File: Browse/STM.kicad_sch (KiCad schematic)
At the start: 2 parts

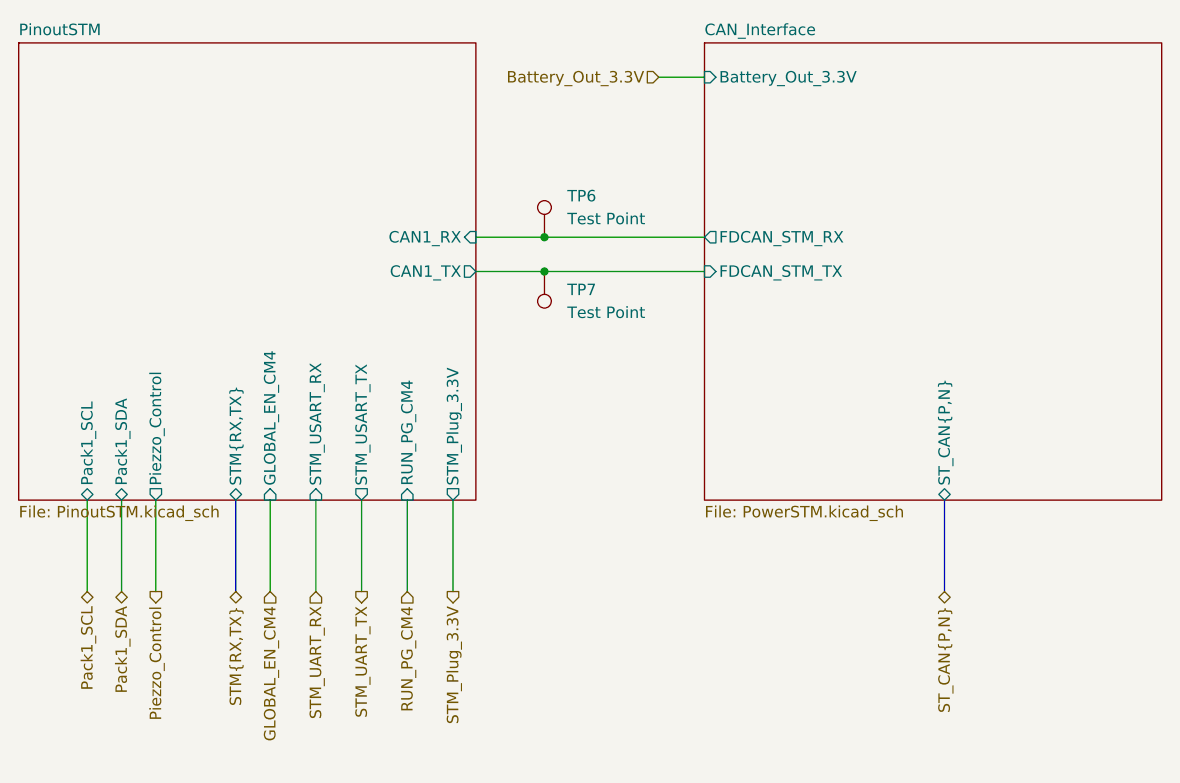
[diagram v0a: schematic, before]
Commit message: Deploying to gh-pages from @ Nautilus-UUV/nautilus-mainboard-PCB@5f5fdd9436d408a604bb268d740c0ac7ce1f5af5 🚀
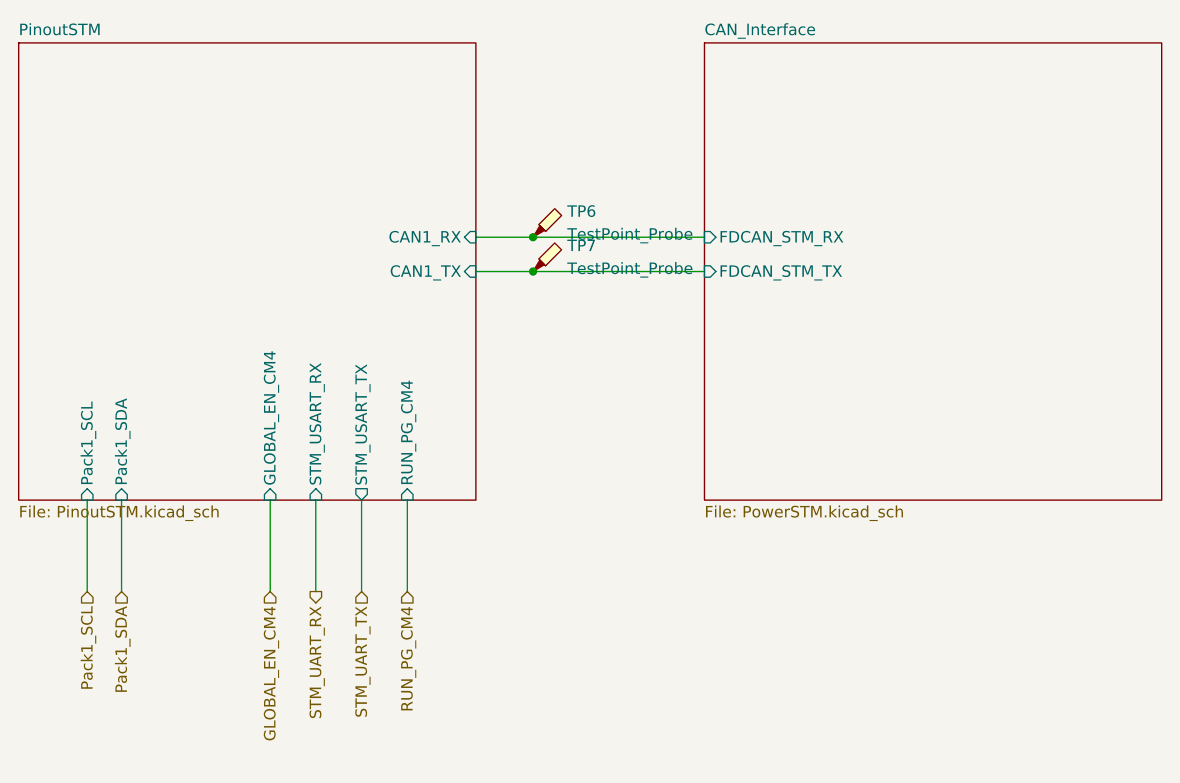
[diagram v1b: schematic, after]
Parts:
- removed TP6, TP7: Test Point, TestPoint:TestPoint_Pad_D1.5mm, symbol #dzdb:g_mech/M-TEST-SMT_1.5mm_round
- added TP6, TP7: TestPoint_Probe, TestPoint:TestPoint_THTPad_D2.5mm_Drill1.2mm, symbol Connector:TestPoint_Probe
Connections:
- net CAN_Interface/FDCAN_STM_RX: now also TP6.1
- net CAN_Interface/FDCAN_STM_TX: now also TP7.1
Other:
- sheet CAN_Interface ports: added none; removed Battery_Out_3.3V, ST_CAN{P,N}
- sheet PinoutSTM ports: added none; removed Piezzo_Control, STM_Plug_3.3V, STM{RX,TX}
- company: Evan -> (none)
- title: Nautilus_Mainboard -> (none)
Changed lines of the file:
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@@
 (kicad_sch (version 20250114) (generator "eeschema") (generator_version "9.0")
   (paper "A4")
-  (title_block
-    (title "Nautilus_Mainboard")
-    (date "2025-11-19")
-    (rev "0")
-    (company "Evan")
+  (junction (at 82.55 50.8) (diameter 0) (color 0 0 0 0)
   )
-  (junction (at 83.82 46.99) (diameter 0) (color 0 0 0 0)
+  (junction (at 82.55 46.99) (diameter 0) (color 0 0 0 0)
   )
-  (junction (at 83.82 50.8) (diameter 0) (color 0 0 0 0)
+  (wire (pts (xy 76.2 46.99) (xy 82.55 46.99))
+    (stroke (width 0) (type default))
   )
   (wire (pts (xy 63.5 76.2) (xy 63.5 86.36))
-    (stroke (width 0) (type default))
-  )
-  (bus (pts (xy 49.53 76.2) (xy 49.53 86.36))
-    (stroke (width 0) (type default))
-  )
-  (wire (pts (xy 40.64 76.2) (xy 40.64 86.36))
     (stroke (width 0) (type default))
   )
@@
     (stroke (width 0) (type default))
   )
-  (wire (pts (xy 73.66 76.2) (xy 73.66 86.36))
+  (wire (pts (xy 76.2 50.8) (xy 82.55 50.8))
     (stroke (width 0) (type default))
   )
-  (wire (pts (xy 76.2 46.99) (xy 83.82 46.99))
+  (wire (pts (xy 82.55 46.99) (xy 101.6 46.99))
     (stroke (width 0) (type default))
   )
@@
     (stroke (width 0) (type default))
   )
-  (wire (pts (xy 83.82 46.99) (xy 101.6 46.99))
-    (stroke (width 0) (type default))
-  )
   (wire (pts (xy 58.42 76.2) (xy 58.42 86.36))
     (stroke (width 0) (type default))
   )
-  (wire (pts (xy 83.82 50.8) (xy 101.6 50.8))
-    (stroke (width 0) (type default))
-  )
-  (bus (pts (xy 128.27 76.2) (xy 128.27 86.36))
-    (stroke (width 0) (type default))
-  )
-  (wire (pts (xy 96.52 29.21) (xy 101.6 29.21))
-    (stroke (width 0) (type default))
-  )
-  (wire (pts (xy 76.2 50.8) (xy 83.82 50.8))
+  (wire (pts (xy 82.55 50.8) (xy 101.6 50.8))
     (stroke (width 0) (type default))
   )
@@
     (stroke (width 0) (type default))
   )
-  (hierarchical_label "STM_UART_TX" (shape output) (at 63.5 86.36 270)
+  (hierarchical_label "STM_UART_TX" (shape input) (at 63.5 86.36 270)
     (effects (font (size 1.27 1.27)) (justify right))
   )
-  (hierarchical_label "STM_UART_RX" (shape input) (at 58.42 86.36 270)
+  (hierarchical_label "STM_UART_RX" (shape output) (at 58.42 86.36 270)
     (effects (font (size 1.27 1.27)) (justify right))
   )
@@
     (effects (font (size 1.27 1.27)) (justify right))
   )
-  (hierarchical_label "Pack1_SCL" (shape bidirectional) (at 33.02 86.36 270)
+  (hierarchical_label "Pack1_SCL" (shape input) (at 33.02 86.36 270)
     (effects (font (size 1.27 1.27)) (justify right))
   )
-  (hierarchical_label "STM{RX,TX}" (shape bidirectional) (at 49.53 86.36 270)
-    (effects (font (size 1.27 1.27)) (justify right))
-  )
-  (hierarchical_label "Battery_Out_3.3V" (shape input) (at 96.52 29.21 180)
-    (effects (font (size 1.27 1.27)) (justify right))
-  )
-  (hierarchical_label "STM_Plug_3.3V" (shape output) (at 73.66 86.36 270)
-    (effects (font (size 1.27 1.27)) (justify right))
-  )
-  (hierarchical_label "Piezzo_Control" (shape output) (at 40.64 86.36 270)
-    (effects (font (size 1.27 1.27)) (justify right))
-  )
-  (hierarchical_label "Pack1_SDA" (shape bidirectional) (at 36.83 86.36 270)
+  (hierarchical_label "Pack1_SDA" (shape input) (at 36.83 86.36 270)
     (effects (font (size 1.27 1.27)) (justify right))
   )
@@
     (effects (font (size 1.27 1.27)) (justify right))
   )
-  (hierarchical_label "ST_CAN{P,N}" (shape bidirectional) (at 128.27 86.36 270)
-    (effects (font (size 1.27 1.27)) (justify right))
-  )
-  (symbol (lib_id "#dzdb:g_mech/M-TEST-SMT_1.5mm_round") (at 83.82 46.99 0) (unit 1)
+  (symbol (lib_id "Connector:TestPoint_Probe") (at 82.55 46.99 0) (unit 1)
     (exclude_from_sim no) (in_bom yes) (on_board yes) (dnp no) (fields_autoplaced)
-    (property "Reference" "TP6" (at 86.36 42.4179 0)
+    (property "Reference" "TP6" (at 86.36 44.1324 0)
       (effects (font (size 1.27 1.27)) (justify left))
     )
-    (property "Value" "Test Point" (at 86.36 44.9579 0)
+    (property "Value" "TestPoint_Probe" (at 86.36 46.6724 0)
       (effects (font (size 1.27 1.27)) (justify left))
     )
-    (property "Footprint" "TestPoint:TestPoint_Pad_D1.5mm" (at 88.9 46.99 0)
+    (property "Footprint" "TestPoint:TestPoint_THTPad_D2.5mm_Drill1.2mm" (at 87.63 46.99 0)
       (effects (font (size 1.27 1.27)) (hide yes))
     )
-    (property "Datasheet" "~" (at 88.9 46.99 0)
+    (property "Datasheet" "~" (at 87.63 46.99 0)
       (effects (font (size 1.27 1.27)) (hide yes))
     )
-    (property "Description" "SMT Test Point 1.5mm round" (at 83.82 46.99 0)
-      (effects (font (size 1.27 1.27)) (hide yes))
-    )
-    (property "IPN" "M-TEST-SMT_1.5mm_round" (at 83.82 46.99 0)
-      (effects (font (size 1.27 1.27)) (hide yes))
-    )
-    (property "Comments" "TestPoint 1.5mm" (at 83.82 46.99 0)
+    (property "Description" "test point (alternative probe-style design)" (at 82.55 46.99 0)
       (effects (font (size 1.27 1.27)) (hide yes))
     )
@@
     )
   )
-  (symbol (lib_id "#dzdb:g_mech/M-TEST-SMT_1.5mm_round") (at 83.82 50.8 180) (unit 1)
+  (symbol (lib_id "Connector:TestPoint_Probe") (at 82.55 50.8 0) (unit 1)
     (exclude_from_sim no) (in_bom yes) (on_board yes) (dnp no) (fields_autoplaced)
-    (property "Reference" "TP7" (at 86.36 52.8319 0)
-      (effects (font (size 1.27 1.27)) (justify right))
+    (property "Reference" "TP7" (at 86.36 47.9424 0)
+      (effects (font (size 1.27 1.27)) (justify left))
     )
-    (property "Value" "Test Point" (at 86.36 55.3719 0)
-      (effects (font (size 1.27 1.27)) (justify right))
+    (property "Value" "TestPoint_Probe" (at 86.36 50.4824 0)
+      (effects (font (size 1.27 1.27)) (justify left))
     )
-    (property "Footprint" "TestPoint:TestPoint_Pad_D1.5mm" (at 78.74 50.8 0)
+    (property "Footprint" "TestPoint:TestPoint_THTPad_D2.5mm_Drill1.2mm" (at 87.63 50.8 0)
       (effects (font (size 1.27 1.27)) (hide yes))
     )
-    (property "Datasheet" "~" (at 78.74 50.8 0)
+    (property "Datasheet" "~" (at 87.63 50.8 0)
       (effects (font (size 1.27 1.27)) (hide yes))
     )
-    (property "Description" "SMT Test Point 1.5mm round" (at 83.82 50.8 0)
-      (effects (font (size 1.27 1.27)) (hide yes))
-    )
-    (property "IPN" "M-TEST-SMT_1.5mm_round" (at 83.82 50.8 0)
-      (effects (font (size 1.27 1.27)) (hide yes))
-    )
-    (property "Comments" "TestPoint 1.5mm" (at 83.82 50.8 0)
+    (property "Description" "test point (alternative probe-style design)" (at 82.55 50.8 0)
       (effects (font (size 1.27 1.27)) (hide yes))
     )
@@
       (effects (font (size 1.27 1.27)) (justify left top))
     )
-    (pin "FDCAN_STM_RX" output (at 101.6 46.99 180)
+    (pin "FDCAN_STM_RX" input (at 101.6 46.99 180)
       (effects (font (size 1.27 1.27)) (justify left))
     )
     (pin "FDCAN_STM_TX" input (at 101.6 50.8 180)
-      (effects (font (size 1.27 1.27)) (justify left))
-    )
-    (pin "Battery_Out_3.3V" input (at 101.6 29.21 180)
-      (effects (font (size 1.27 1.27)) (justify left))
-    )
-    (pin "ST_CAN{P,N}" bidirectional (at 128.27 76.2 270)
       (effects (font (size 1.27 1.27)) (justify left))
     )
@@
       (effects (font (size 1.27 1.27)) (justify right))
     )
+    (pin "CAN1_TX" input (at 76.2 50.8 0)
+      (effects (font (size 1.27 1.27)) (justify right))
+    )
     (pin "STM_USART_RX" input (at 58.42 76.2 270)
       (effects (font (size 1.27 1.27)) (justify left))
@@
       (effects (font (size 1.27 1.27)) (justify left))
     )
-    (pin "CAN1_TX" output (at 76.2 50.8 0)
-      (effects (font (size 1.27 1.27)) (justify right))
-    )
-    (pin "Pack1_SCL" bidirectional (at 33.02 76.2 270)
+    (pin "Pack1_SCL" input (at 33.02 76.2 270)
       (effects (font (size 1.27 1.27)) (justify left))
     )
-    (pin "Pack1_SDA" bidirectional (at 36.83 76.2 270)
+    (pin "Pack1_SDA" input (at 36.83 76.2 270)
       (effects (font (size 1.27 1.27)) (justify left))
     )
-    (pin "STM_Plug_3.3V" output (at 73.66 76.2 270)
-      (effects (font (size 1.27 1.27)) (justify left))
-    )
-    (pin "Piezzo_Control" output (at 40.64 76.2 270)
-      (effects (font (size 1.27 1.27)) (justify left))
-    )
-    (pin "STM{RX,TX}" bidirectional (at 49.53 76.2 270)
-      (effects (font (size 1.27 1.27)) (justify left))
-    )
